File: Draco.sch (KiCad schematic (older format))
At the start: 51 parts, among them J1 Conn_01x03, J10 Conn_01x03, J11 Conn_01x06, J12 Conn_02x05_Odd_Even, J13 Conn_01x04, J14 Conn_01x01, J15 Micro_SD_Card, J2 Conn_01x03, J20 Conn_01x04, J3 Conn_01x03, J4 Conn_01x03, J5 Conn_01x03, J6 Conn_01x03, J7 Conn_01x03, J8 Conn_01x03, J9 Conn_01x03, U1 ATMEGA2560-16AU, U2 LOGIC-TXS0108EPWR(TSSOP20), U3 RFM95HW, Y1 16MHz

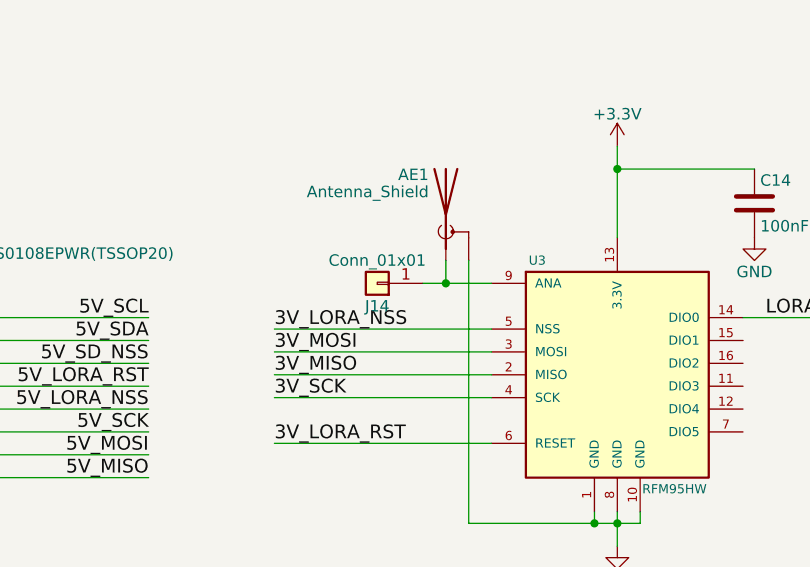
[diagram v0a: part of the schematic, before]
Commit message: Finished left side
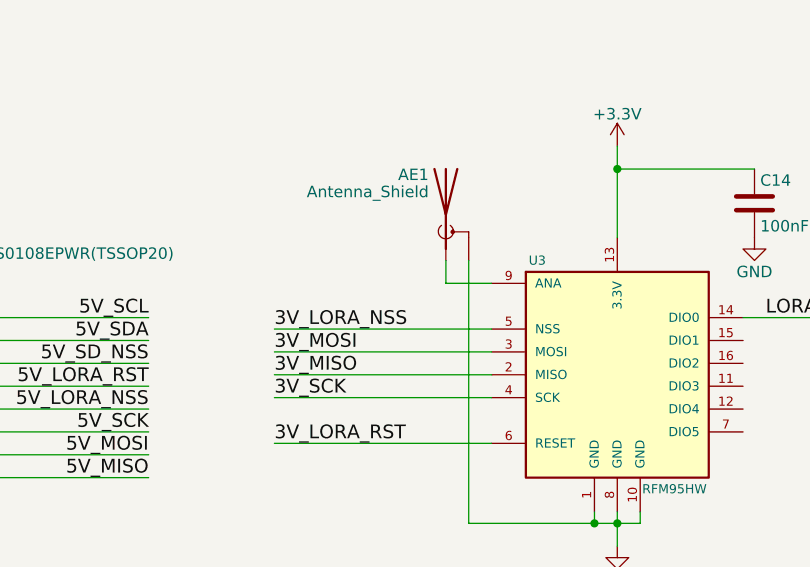
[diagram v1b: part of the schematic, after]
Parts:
- removed J14: Conn_01x01, Pin_Headers:Pin_Header_Straight_1x01_Pitch2.54mm, symbol Conn_01x01
- J11: footprint Connectors_JST:JST_PH_B6B-PH-K_06x2.00mm_Straight -> Socket_Strips:Socket_Strip_Straight_1x06_Pitch2.54mm
- J13: footprint Connectors_JST:JST_PH_B4B-PH-K_04x2.00mm_Straight -> Connectors_JST:JST_XH_B04B-XH-A_04x2.50mm_Straight
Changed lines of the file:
@@
 F 0 "J11" H 7800 9450 50  0000 C CNN
 F 1 "Conn_01x06" H 7800 8750 50  0000 C CNN
-F 2 "Connectors_JST:JST_PH_B6B-PH-K_06x2.00mm_Straight" H 7800 9150 50  0001 C CNN
+F 2 "Socket_Strips:Socket_Strip_Straight_1x06_Pitch2.54mm" H 7800 9150 50  0001 C CNN
 F 3 "" H 7800 9150 50  0001 C CNN
 	1    7800 9150
@@
 	1    0    0    -1
 $EndComp
-$Comp
-L Conn_01x01 J14
-U 1 1 5A5F4C41
-P 14100 7450
-F 0 "J14" H 14100 7550 50  0000 C CNN
-F 1 "Conn_01x01" H 14100 7350 50  0000 C CNN
-F 2 "Pin_Headers:Pin_Header_Straight_1x01_Pitch2.54mm" H 14100 7450 50  0001 C CNN
-F 3 "" H 14100 7450 50  0001 C CNN
-	1    14100 7450
-	-1   0    0    1
-$EndComp
 Text Label 8050 2800 2    60   ~ 0
 5V_LORA_NSS
@@
 F 0 "J13" H 12150 5300 50  0000 C CNN
 F 1 "Conn_01x04" H 12150 4800 50  0000 C CNN
-F 2 "Connectors_JST:JST_PH_B4B-PH-K_04x2.00mm_Straight" H 12150 5100 50  0001 C CNN
+F 2 "Connectors_JST:JST_XH_B04B-XH-A_04x2.50mm_Straight" H 12150 5100 50  0001 C CNN
 F 3 "" H 12150 5100 50  0001 C CNN
 	1    12150 5100
@@
 	14500 7350 14500 8500
 Connection ~ 15050 8500
-Wire Wire Line
-	14300 7450 14600 7450
-Wire Wire Line
-	14400 7450 14400 7350
-Connection ~ 14400 7450
 Wire Wire Line
 	7400 2400 8050 2400
@@
 	1    0    0    -1
 $EndComp
+Wire Wire Line
+	14600 7450 14400 7450
+Wire Wire Line
+	14400 7450 14400 7350
 $EndSCHEMATC
